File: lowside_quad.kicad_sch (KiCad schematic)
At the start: 4 parts, among them U2 1k, U3 1k, U4 VNLD5160, U5 VNLD5160

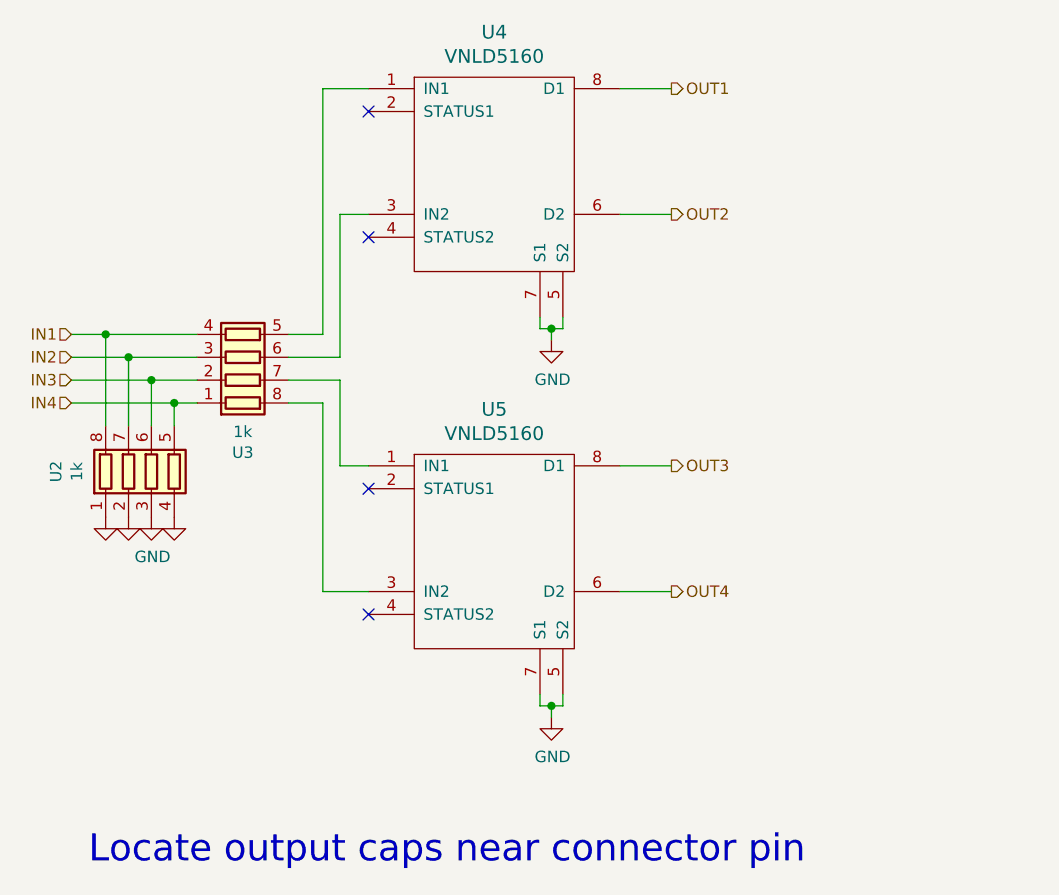
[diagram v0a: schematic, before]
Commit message: Upd SCH
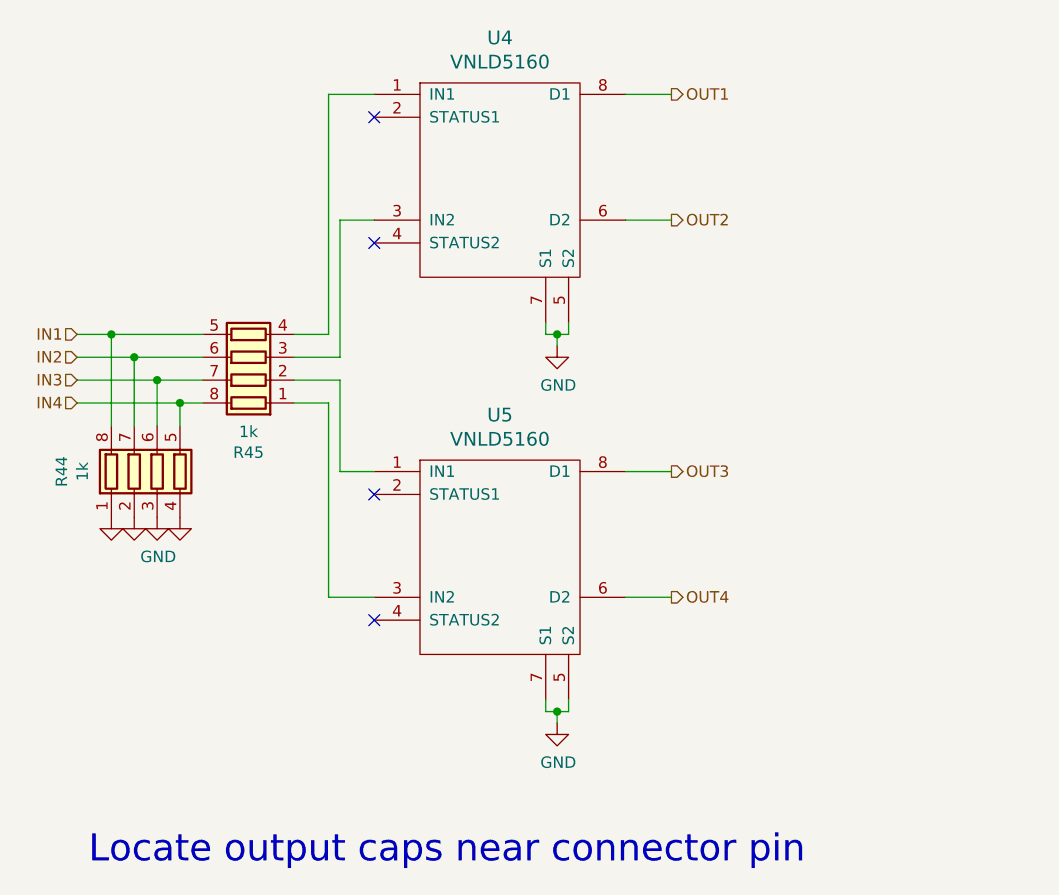
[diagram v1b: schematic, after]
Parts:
- renumbered U2 to R44, U3 to R45
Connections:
- net IN1: now also R45.5 (R4.2); no longer R45.4 (R4.1)
- net IN2: now also R45.6 (R3.2); no longer R45.3 (R3.1)
- net IN3: now also R45.7 (R2.2); no longer R45.2 (R2.1)
- net IN4: now also R45.8 (R1.2); no longer R45.1 (R1.1)
- net at U4.1 (IN1): now also R45.4 (R4.1); no longer R45.5 (R4.2)
- net at U4.3 (IN2): now also R45.3 (R3.1); no longer R45.6 (R3.2)
- net at U5.1 (IN1): now also R45.2 (R2.1); no longer R45.7 (R2.2)
- net at U5.3 (IN2): now also R45.1 (R1.1); no longer R45.8 (R1.2)
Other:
- moved on the sheet: R44, R45, U4, U5

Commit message: Export
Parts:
- U4, U5: LCSC N/A -> C377942
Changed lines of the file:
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@@
       (effects (font (size 1.27 1.27)) hide)
     )
-    (property "LCSC" "N/A" (at 106.68 52.07 0)
+    (property "LCSC" "C377942" (at 106.68 52.07 0)
       (effects (font (size 1.27 1.27)) hide)
     )
@@
       (effects (font (size 1.27 1.27)) hide)
     )
-    (property "LCSC" "N/A" (at 106.68 93.98 0)
+    (property "LCSC" "C377942" (at 106.68 93.98 0)
       (effects (font (size 1.27 1.27)) hide)
     )
